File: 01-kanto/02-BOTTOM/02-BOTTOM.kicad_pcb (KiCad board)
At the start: 2 copper layers, 44 x 25 mm, 31 parts, among them J2 Conn_01x04, J3 USB_C_Receptacle_USB2.0_16P, SW1 SW_Push, SW2 SW_Push, U3 STM32F103C8Tx, U4 CH340E, U5 AMS1117-3.3

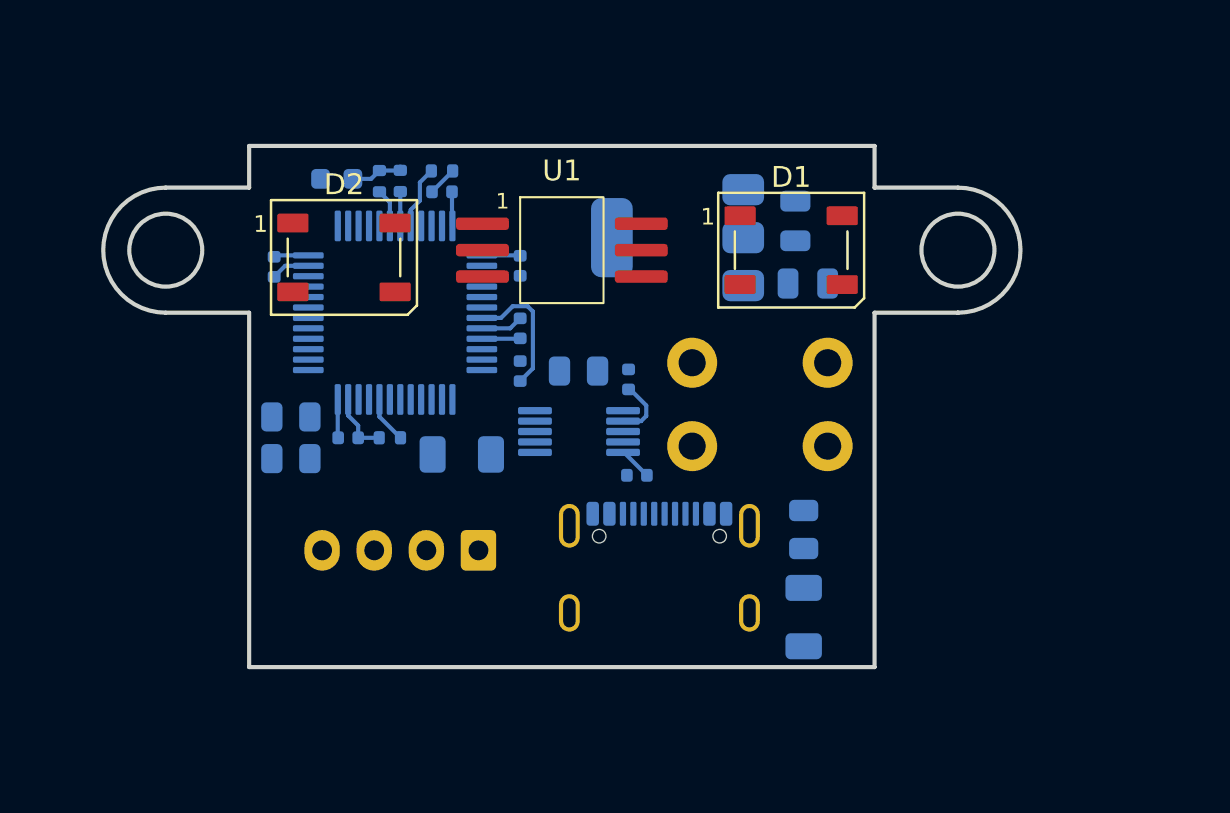
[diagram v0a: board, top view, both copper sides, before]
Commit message: 02-BOTTOM PCBdesign completed
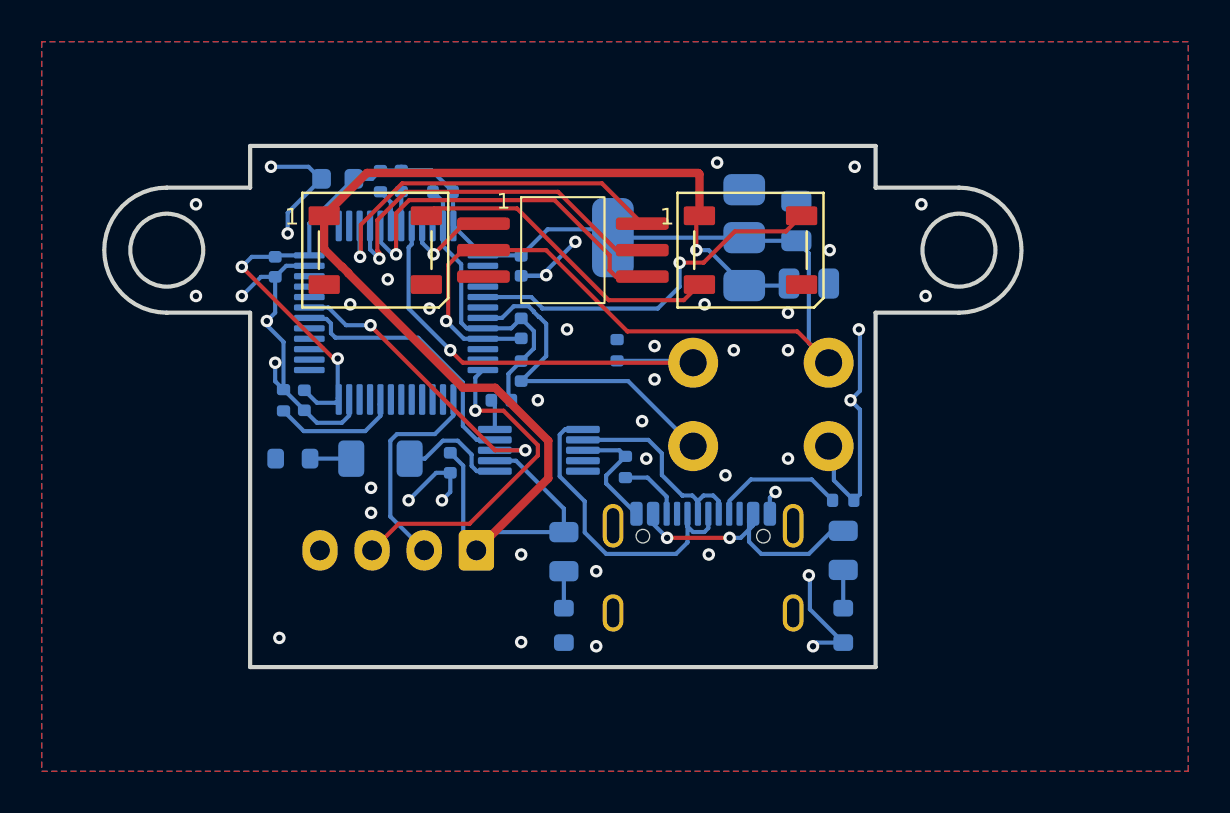
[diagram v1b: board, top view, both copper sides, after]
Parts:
- added D5: LED_GREEN, LED_SMD:LED_0805_2012Metric, B.Cu at (120.0, 84.5)
- added R9: 470, Resistor_SMD:R_0603_1608Metric, B.Cu at (120.0, 88.0)
- D3: footprint LED_SMD:LED_1206_3216Metric -> LED_SMD:LED_0805_2012Metric
- D4: value LED_ORANGE -> LED_YELLOW
- R1, R3: footprint Resistor_SMD:R_0805_2012Metric -> Resistor_SMD:R_0402_1005Metric
- R2, R4: value 75 -> 470; footprint Resistor_SMD:R_0805_2012Metric -> Resistor_SMD:R_0603_1608Metric
- moved R3 26.6 mm to (133.4, 82.0), turned to 180 degrees
- moved R1 16.2 mm to (123.0, 80.4), turned to -90 degrees
- moved R4 14.3 mm to (107.0, 80.0), turned to 180 degrees
- moved R6 12.0 mm to (122.6, 74.8), turned to 90 degrees
- moved C2 9.44 mm to (114.6, 80.2), turned to 90 degrees
- moved C1 7.43 mm to (117.0, 77.2), turned to 0 degrees
- moved R5 5.41 mm to (106.6, 77.2), turned to 90 degrees
- moved R2 4.98 mm to (133.4, 88.0), turned to -90 degrees
- moved D4 3.91 mm to (111.2, 80.0), turned to 0 degrees
- moved D3 3.72 mm to (133.4, 84.4), turned to 90 degrees
- moved C5 2.77 mm to (107.6, 77.2), turned to -90 degrees
- moved U4 2.13 mm to (118.8, 79.6), turned to 180 degrees
- moved J3 2.10 mm to (126.7, 86.3)
- moved D1 1.95 mm to (129.0, 70.0)
- moved D2 1.54 mm to (111.0, 70.0)
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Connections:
- U1 pad 2: +5V -> +3V3
- U3 pad 22: CS_Dout -> unconnected-(U3-PB11-Pad22)
- U3 pad 25: CS_Range -> unconnected-(U3-PB12-Pad25)
- U3 pad 26: CS_CK -> unconnected-(U3-PB13-Pad26)
- U3 pad 27: CS_Gate -> unconnected-(U3-PB14-Pad27)
- U3 pad 28: LED -> unconnected-(U3-PB15-Pad28)
- U3 pad 39: unconnected-(U3-PB3-Pad39) -> CS_Gate
- U3 pad 40: unconnected-(U3-PB4-Pad40) -> CS_CK
- U3 pad 41: unconnected-(U3-PB5-Pad41) -> CS_Range
- U3 pad 45: unconnected-(U3-PB8-Pad45) -> CS_Dout
- U3 pad 5: unconnected-(U3-PD0-Pad5) -> LED
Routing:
- net +3V3: track 11.3 -> 77.2 mm, vias 0 -> 3
- net +5V: track 2.89 -> 65.8 mm, vias 0 -> 1
- net GND: track 8.35 -> 69.5 mm, vias 0 -> 44
- net BOOT0: track 3.05 -> 22.4 mm, vias 0 -> 1
- net CS_CK: track 0.00 -> 18.7 mm, vias 0 -> 1
- net CS_Gate: track 0.00 -> 18.2 mm, vias 0 -> 1
- net LED: track 0.00 -> 18.0 mm, vias 0 -> 1
- net CS_Range: track 0.00 -> 17.8 mm, vias 0 -> 1
- net UART2_TX: track 0.00 -> 16.1 mm, vias 0 -> 1
- net D+: track 0.00 -> 15.9 mm
- net Net-(D1-DOUT): track 0.00 -> 15.4 mm
- net UART1_RX: track 0.00 -> 14.7 mm, vias 0 -> 2
- net Net-(D3-A): track 0.00 -> 13.4 mm, vias 0 -> 2
- net UART1_TX: track 0.00 -> 12.8 mm
- net UART2_RX: track 0.00 -> 10.2 mm
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- added copper zone on B.Cu, net GND
- added copper zone on F.Cu, net GND
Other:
- outline, holes or cut-outs redrawn
